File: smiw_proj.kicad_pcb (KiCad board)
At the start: 2 copper layers, 115.6 x 104.1 mm, 60 parts, among them J1 Conn_02x06_Odd_Even, J2 Conn_02x05_Odd_Even, J3 Conn_01x02, J4 Conn_01x02, J5 Conn_02x05_Odd_Even, J6 Molex 104031, J7 Conn_02x06_Odd_Even, M1 JGB37-520, SW1 SW_Push, U1 LM2596S-5, U2 M5 Stamp-S3, U3 LD1117S33TR_SOT223, U4 L298N

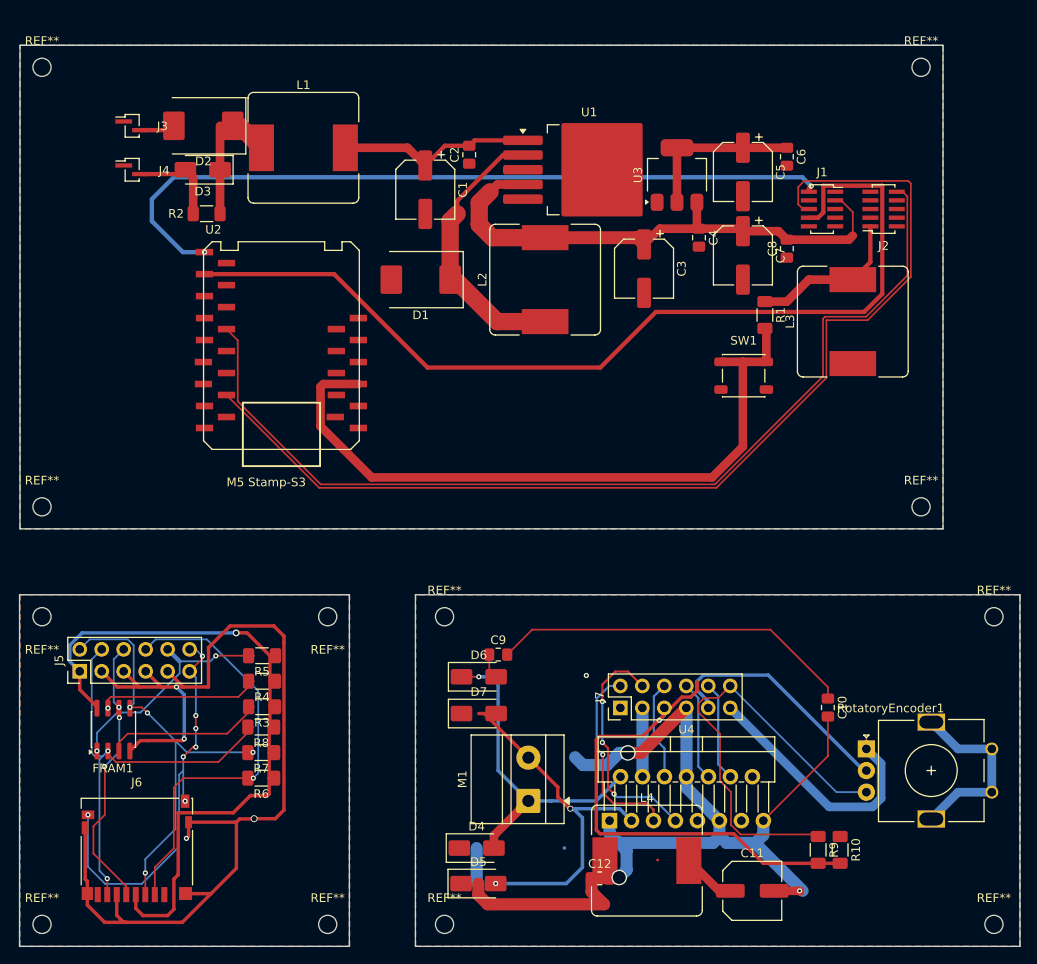
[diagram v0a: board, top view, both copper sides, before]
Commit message: pcb dobrze zdaniem michala (to nie ma sensu)
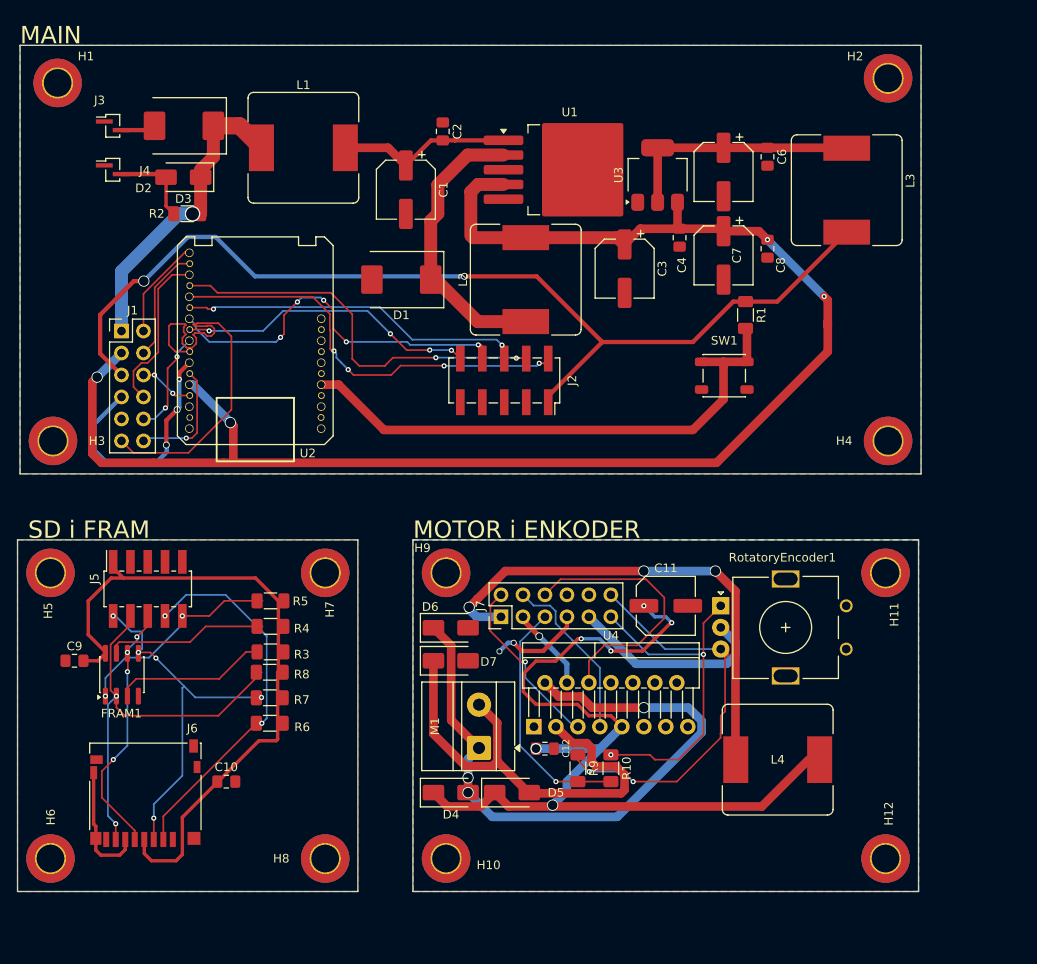
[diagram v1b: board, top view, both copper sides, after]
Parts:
- removed REF** (x12): MountingHole_2.1mm, MountingHole:MountingHole_2.1mm
- added H1: MountingHole, MountingHole:MountingHole_3.2mm_M3_DIN965_Pad_TopBottom, F.Cu at (19.6, 17.0)
- added H10: MountingHole, MountingHole:MountingHole_3.2mm_M3_DIN965_Pad_TopBottom, F.Cu at (64.5, 106.7)
- added H11: MountingHole, MountingHole:MountingHole_3.2mm_M3_DIN965_Pad_TopBottom, F.Cu at (115.3, 73.7)
- added H12: MountingHole, MountingHole:MountingHole_3.2mm_M3_DIN965_Pad_TopBottom, F.Cu at (115.3, 106.7)
- added H2: MountingHole, MountingHole:MountingHole_3.2mm_M3_DIN965_Pad_TopBottom, F.Cu at (115.6, 16.5)
- added H3: MountingHole, MountingHole:MountingHole_3.2mm_M3_DIN965_Pad_TopBottom, F.Cu at (19.1, 58.4)
- added H4: MountingHole, MountingHole:MountingHole_3.2mm_M3_DIN965_Pad_TopBottom, F.Cu at (115.6, 58.4)
- added H5: MountingHole, MountingHole:MountingHole_3.2mm_M3_DIN965_Pad_TopBottom, F.Cu at (18.8, 73.7)
- added H6: MountingHole, MountingHole:MountingHole_3.2mm_M3_DIN965_Pad_TopBottom, F.Cu at (18.8, 106.7)
- added H7: MountingHole, MountingHole:MountingHole_3.2mm_M3_DIN965_Pad_TopBottom, F.Cu at (50.5, 73.7)
- added H8: MountingHole, MountingHole:MountingHole_3.2mm_M3_DIN965_Pad_TopBottom, F.Cu at (50.5, 106.7)
- added H9: MountingHole, MountingHole:MountingHole_3.2mm_M3_DIN965_Pad_TopBottom, F.Cu at (64.5, 73.7)
- J1: footprint Connector_PinSocket_1.00mm:PinSocket_2x05_P1.00mm_Vertical_SMD -> Connector_PinHeader_2.54mm:PinHeader_2x06_P2.54mm_Vertical
- J2: footprint Connector_PinSocket_1.00mm:PinSocket_2x05_P1.00mm_Vertical_SMD -> Connector_PinSocket_2.54mm:PinSocket_2x05_P2.54mm_Vertical_SMD
- J5: footprint Connector_PinHeader_2.54mm:PinHeader_2x06_P2.54mm_Vertical -> Connector_PinSocket_2.00mm:PinSocket_2x05_P2.00mm_Vertical_SMD
- U2: footprint Library2:Stamp-S3_PIN1.27_Socket -> Library:M5Stamp-S3
- moved J1 82.2 mm to (27.0, 45.7)
- moved C10 70.1 mm to (39.1, 97.8), turned to 0 degrees
- moved C9 49.0 mm to (21.5, 83.8)
- moved J2 48.1 mm to (71.2, 51.4), turned to -90 degrees
- moved C11 34.4 mm to (89.9, 77.5)
- moved R9 29.3 mm to (79.7, 96.2)
- moved R10 28.1 mm to (83.5, 96.2)
- moved RotatoryEncoder1 23.6 mm to (96.2, 77.5)
- moved L4 19.1 mm to (102.8, 95.3)
- moved J7 17.4 mm to (70.8, 78.8)
- moved C12 16.3 mm to (75.9, 94.0)
- moved L3 15.2 mm to (110.8, 29.4), turned to -90 degrees
- moved U2 15.0 mm to (43.0, 32.6)
- moved U4 13.9 mm to (74.6, 91.5)
- moved J5 12.3 mm to (30.0, 75.5)
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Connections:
- net //FRAM CS renamed /~{FRAM_CS_2}
- net //SD CS renamed /~{SD_CS_2}
- net VDD renamed VDD_2
- C10 pad 2: GND -> GND_CPU_2
- C11 pad 2: GND -> GND_1
- C12 pad 2: GND -> GND_1
- C9 pad 1: GND -> GND_CPU_2
- D6 pad 2: GND -> GND_1
- D7 pad 2: GND -> GND_1
- FRAM1 pad 2: /MISO -> /MISO_2
- FRAM1 pad 4: GND -> GND_CPU_2
- FRAM1 pad 5: /MOSI -> /MOSI_2
- FRAM1 pad 6: /SCK -> /SCK_2
- J5 pad 2: /MOSI -> /MOSI_2
- J5 pad 3: GND -> GND_CPU_2
- J5 pad 4: /MISO -> /MISO_2
- J5 pad 5: GND -> GND_CPU_2
- J5 pad 6: /SCK -> /SCK_2
- J5 pad 7: GND -> GND_CPU_2
- J5 pad 9: GND -> GND_CPU_2
- J6 pad 3: /MOSI -> /MOSI_2
- J6 pad 5: /SCK -> /SCK_2
- J6 pad 6: GND -> GND_CPU_2
- J6 pad 7: /MISO -> /MISO_2
- J6 pad SH: GND -> GND_CPU_2
- J7 pad 1: 12V -> 12V_1
- J7 pad 10: /DRIVER IN4 -> unconnected-(J7-Pin_10-Pad10)
- J7 pad 11: /ENC A -> /ENC_A_1
- J7 pad 12: /ENC B -> /ENC_B_1
- J7 pad 2: /DRIVER IN1 -> /DRIVER_IN1_1
- J7 pad 3: Vcc -> Vcc_1
- J7 pad 4: /DRIVER IN2 -> /DRIVER_IN2_1
- J7 pad 5: Vdd -> Vdd_1
- J7 pad 6: /PWM A -> /PWM_A_1
- J7 pad 7: GND -> GND_1
- J7 pad 8: /DRIVER IN3 -> unconnected-(J7-Pin_8-Pad8)
- J7 pad 9: CPU_GND -> CPU_GND_1
- L4 pad 1: 12V -> 12V_1
- R10 pad 1: /ENC A -> /ENC_A_1
- R10 pad 2: Vdd -> Vdd_1
- R7 pad 2: /MOSI -> /MOSI_2
- R8 pad 2: /MISO -> /MISO_2
- R9 pad 1: /ENC B -> /ENC_B_1
- R9 pad 2: Vdd -> Vdd_1
- RotatoryEncoder1 pad A: /ENC A -> /ENC_A_1
- RotatoryEncoder1 pad B: /ENC B -> /ENC_B_1
- RotatoryEncoder1 pad C: CPU_GND -> CPU_GND_1
- U4 pad 1: GND -> GND_1
- U4 pad 10: /DRIVER IN3 -> unconnected-(U4-IN3-Pad10)
- U4 pad 11: GND -> GND_1
- U4 pad 12: /DRIVER IN4 -> unconnected-(U4-IN4-Pad12)
- U4 pad 15: GND -> GND_1
- U4 pad 4: Vcc -> Vcc_1
- U4 pad 5: /DRIVER IN1 -> /DRIVER_IN1_1
- U4 pad 6: /PWM A -> /PWM_A_1
- U4 pad 7: /DRIVER IN2 -> /DRIVER_IN2_1
- U4 pad 8: GND -> GND_1
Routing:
- net GND: track 214.7 -> 28.3 mm, vias 7 -> 3
- net /PWM A: track 136.7 -> 6.33 mm, vias 0 -> 2
- net Vcc: track 70.5 -> 180.2 mm, vias 1 -> 4
- net /DRIVER IN3: track 122.2 -> 18.8 mm
- net /DRIVER IN1: track 111.0 -> 11.6 mm, vias 3 -> 0
- net /~{FRAM CS}: track 114.7 -> 34.6 mm, vias 0 -> 4
- net Net-(D4-K): track 30.6 -> 107.6 mm, vias 0 -> 6
- net (no net): track 70.0 -> 0.00 mm, vias 7 -> 0
- net 12V_1: track 0.00 -> 56.0 mm, vias 0 -> 3
- net /MISO_2: track 0.00 -> 48.5 mm, vias 0 -> 2
- net /ENC_B_1: track 0.00 -> 46.2 mm, vias 0 -> 2
- net /~{SD CS}: track 0.00 -> 43.7 mm, vias 0 -> 5
- net VDD_2: track 121.1 -> 77.9 mm, vias 1 -> 0
- net Vdd: track 75.1 -> 117.8 mm, vias 1 -> 2
- net /MOSI_2: track 0.00 -> 42.4 mm, vias 0 -> 5
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- added copper zone on B.Cu, net CPU_GND_1
- added copper zone on F.Cu, net GND_1
- added copper zone on F.Cu, net GND_CPU_2
- removed copper zone on B.Cu, net GND
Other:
- board size 115.6 x 104.1 mm -> 104.4 x 97.8 mm
